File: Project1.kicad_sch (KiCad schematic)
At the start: 50 parts, among them IC1 LM324N, IC2 LM324N, IC3 LM324N, IC4 LM324N

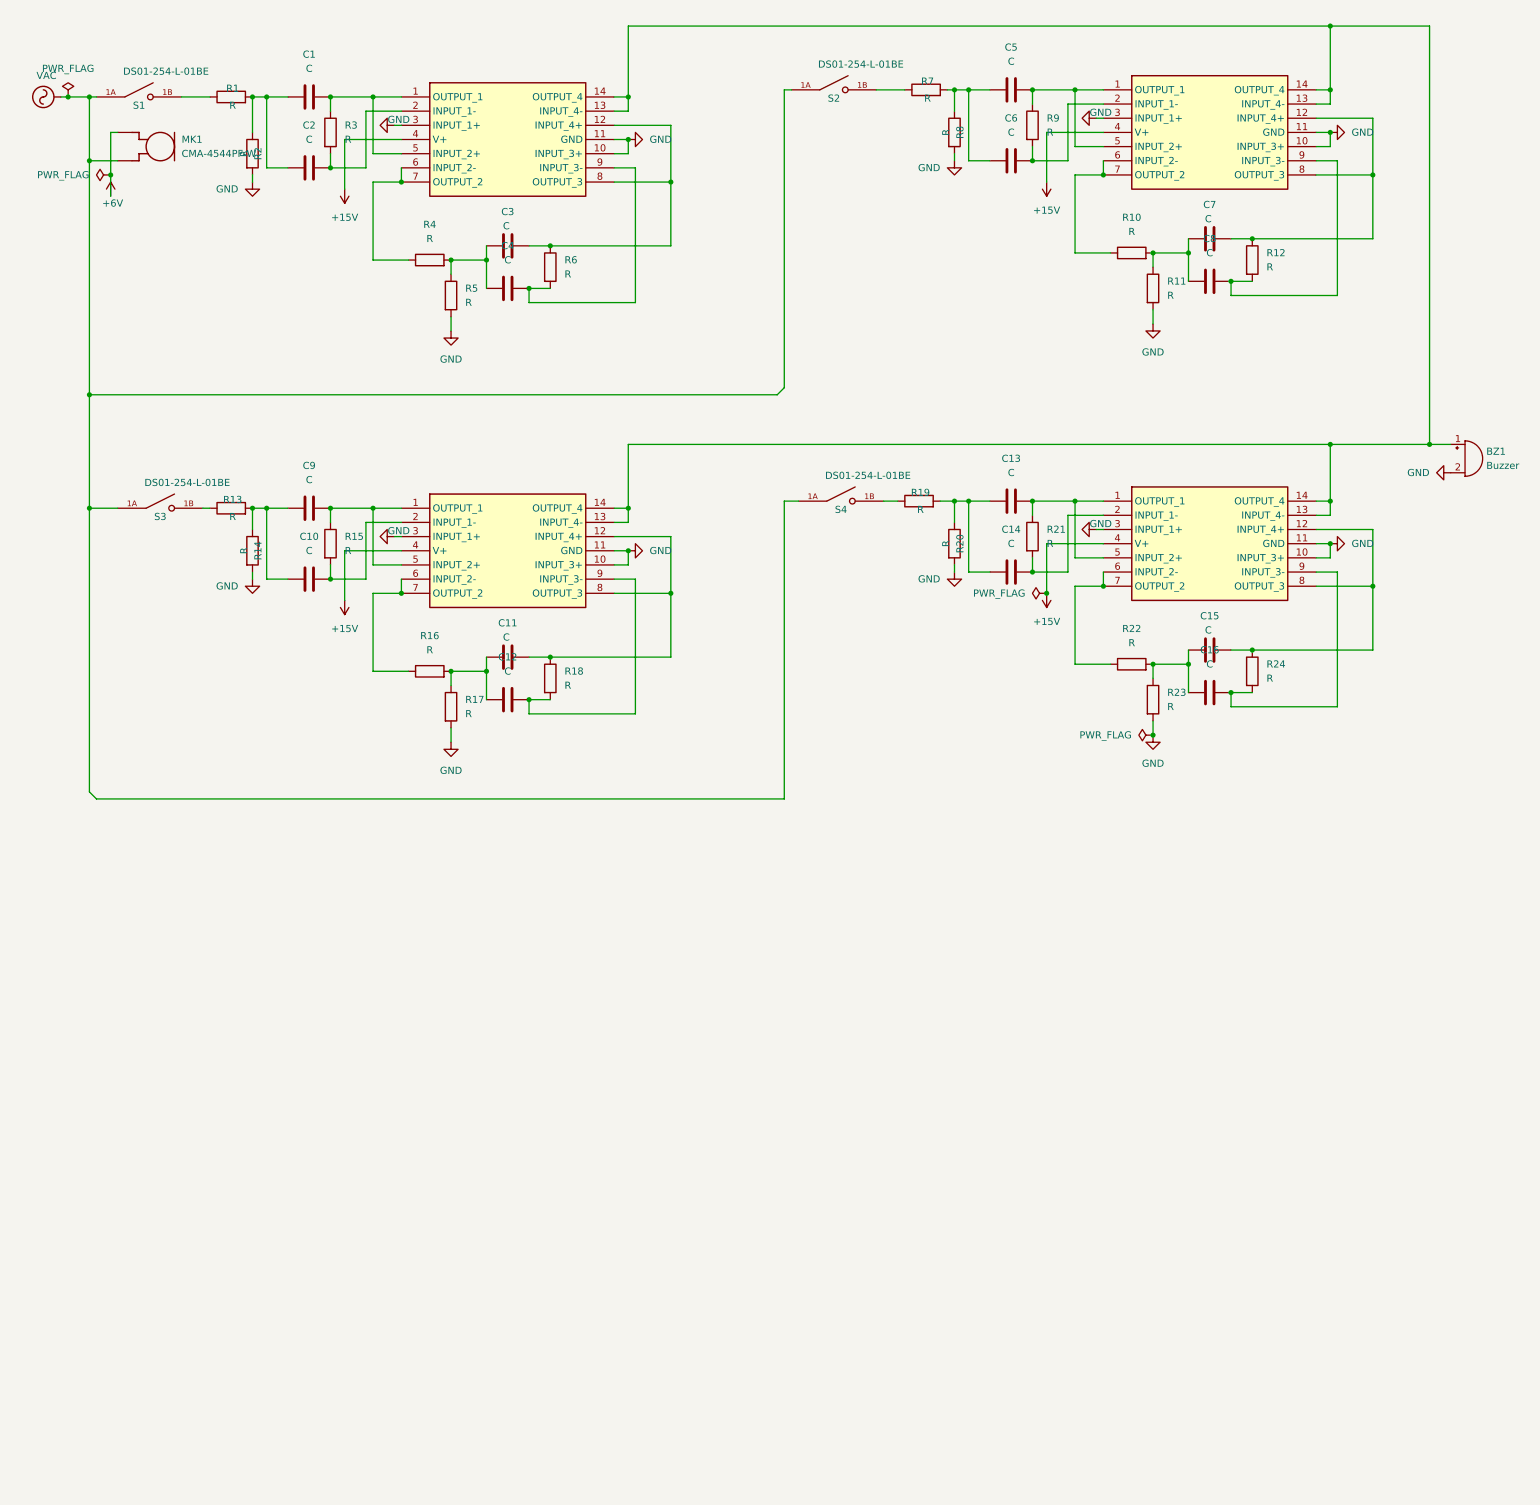
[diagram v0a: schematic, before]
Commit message: 0520 Edited.
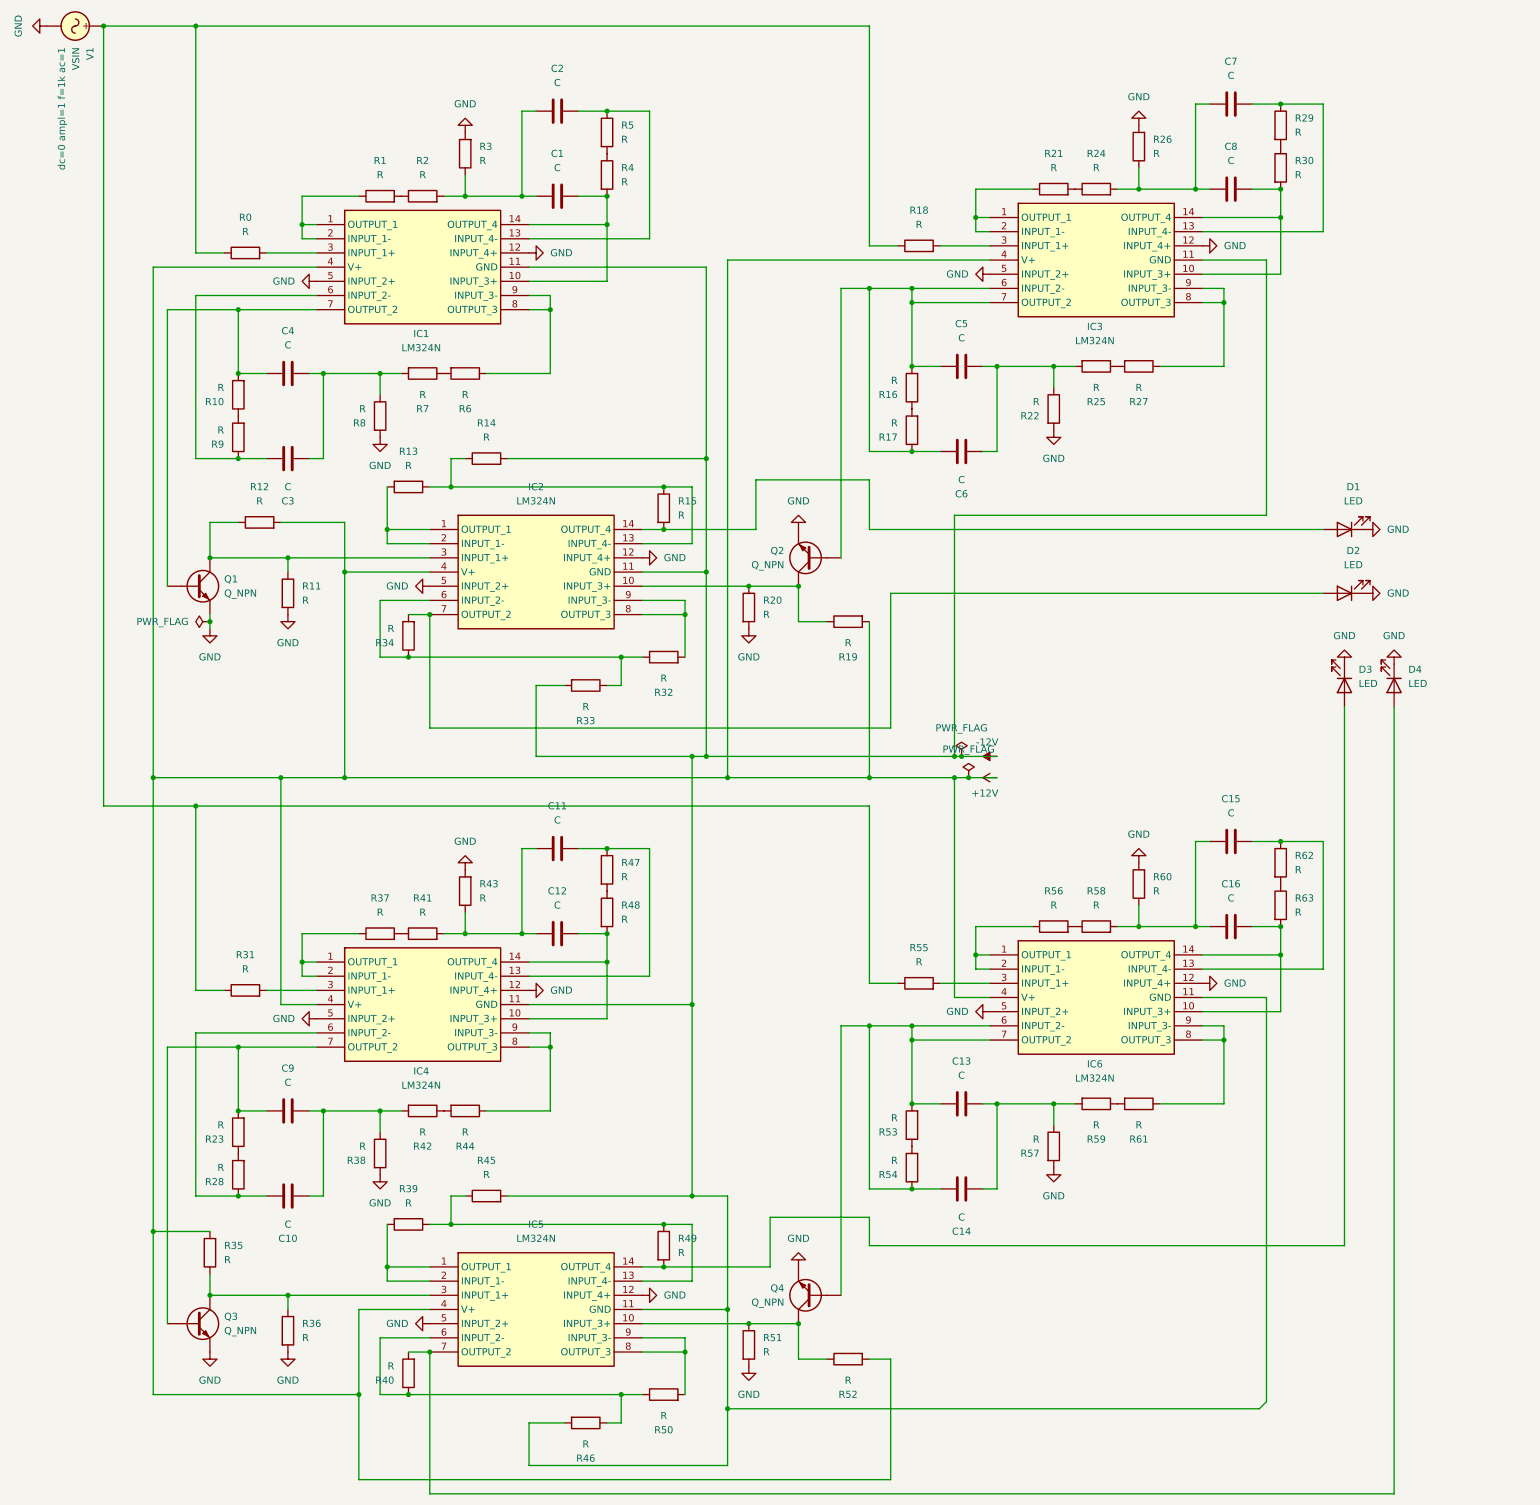
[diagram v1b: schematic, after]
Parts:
- removed BZ1: Buzzer, Buzzer_Beeper:Buzzer_12x9.5RM7.6, symbol Device:Buzzer
- removed MK1: CMA-4544PF-W, Project1:MIC_CMA-4544PF-W, symbol New_Library:CMA-4544PF-W
- removed S1, S2, S3, S4: DS01-254-L-01BE, Project1:SW_DS01-254-L-01BE, symbol New_Library:DS01-254-L-01BE
- added D1, D2, D3, D4: LED, LED_THT:LED_D3.0mm, symbol Device:LED
- added IC5, IC6: LM324N, Project1:LM324N, symbol New_Library:LM324N
- added Q1, Q2, Q3, Q4: Q_NPN, Project1:TNPN_TO-92_ONS, symbol Device:Q_NPN
- added R0, R25, R26, R27, R28, R29, R30, R31, R32, R33, R34, R35, R36, R37, R38, R39, R40, R41, R42, R43, R44, R45, R46, R47, R48, R49, R50, R51, R52, R53, R54, R55, R56, R57, R58, R59, R60, R61, R62, R63: R, Resistor_SMD:R_0603_1608Metric, symbol Device:R
- added V1: VSIN, symbol Simulation_SPICE:VSIN
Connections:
- net GND: now also IC1.12 (INPUT_4+), IC1.5 (INPUT_2+), IC2.12 (INPUT_4+), IC2.5 (INPUT_2+), IC3.12 (INPUT_4+), IC3.5 (INPUT_2+), IC4.12 (INPUT_4+), IC4.5 (INPUT_2+), R22.2, R3.2, D1.1 (K), D2.1 (K), D3.1 (K), D4.1 (K), IC5.12 (INPUT_4+), IC5.5 (INPUT_2+), IC6.12 (INPUT_4+), IC6.5 (INPUT_2+), Q1.E, Q2.E, Q3.E, Q4.E, R26.2, R36.2, R38.2, R43.2, R51.2, R57.2, R60.2, V1.2; no longer IC1.10 (INPUT_3+), IC1.11 (GND), IC1.3 (INPUT_1+), IC2.10 (INPUT_3+), IC2.11 (GND), IC2.3 (INPUT_1+), IC3.10 (INPUT_3+), IC3.11 (GND), IC3.3 (INPUT_1+), IC4.10 (INPUT_3+), IC4.11 (GND), IC4.3 (INPUT_1+), R14.2, R17.2, R2.2, R23.2, R5.2
- net at R1.2, R2.1: no longer C1.2, C2.1
- net at C13.2, C14.1: now also R57.1, R59.2; no longer R19.2, R20.1
- net at IC1.8 (OUTPUT_3), R6.1: now also IC1.9 (INPUT_3-); no longer C3.2, IC1.12 (INPUT_4+)
- net at R7.1: now also R6.2
- net at C5.2, C6.1: now also R22.1, R25.2; no longer R7.2, R8.1
- net at R16.2, R17.1: now also C5.1, C6.2, IC3.6 (INPUT_2-), IC3.7 (OUTPUT_2), Q2.B; no longer C11.1, C12.1
- net at C15.1, C16.1: now also R58.2, R60.1; no longer R22.2, R23.1
- net at R19.1: now also IC2.10 (INPUT_3+), R20.1, Q2.C
- net at R13.1: now also IC2.13 (INPUT_4-), R14.1, R15.1
- net at C10.1, C9.2: now also R38.1, R42.2; no longer R13.2, R14.1
- net at C7.1, C8.1: now also R24.2, R26.1; no longer R10.2, R11.1
- net at R1.1: now also IC1.1 (OUTPUT_1), IC1.2 (INPUT_1-)
- net at C1.1, R3.1: now also C2.1, R2.2; no longer IC1.1 (OUTPUT_1), IC1.5 (INPUT_2+)
- net +15V renamed +12V
- net +12V: now also R12.2, R19.2, IC5.4 (V+), IC6.4 (V+), R35.2, R52.2
- new net: R0.1, R18.1, R31.1, R55.1, V1.1
- new net: IC6.3 (INPUT_1+), R55.2
- new net: IC3.1 (OUTPUT_1), IC3.2 (INPUT_1-), R21.1
- new net: R21.2, R24.1
- new net: IC5.1 (OUTPUT_1), IC5.2 (INPUT_1-), R39.2
- new net: IC5.10 (INPUT_3+), Q4.C, R51.1, R52.1
- new net: IC5.13 (INPUT_4-), R39.1, R45.1, R49.1
- new net: D3.2 (A), IC5.14 (OUTPUT_4), R49.2
- new net: IC5.3 (INPUT_1+), Q3.C, R35.1, R36.1
- new net: IC5.6 (INPUT_2-), R40.1, R46.1, R50.1
- new net: D4.2 (A), IC5.7 (OUTPUT_2), R40.2
- new net: IC5.8 (OUTPUT_3), IC5.9 (INPUT_3-), R50.2
- new net: C7.2, IC3.13 (INPUT_4-), R29.1
- new net: IC2.6 (INPUT_2-), R32.1, R33.1, R34.1
- new net: R29.2, R30.1
- new net: C8.2, IC3.10 (INPUT_3+), IC3.14 (OUTPUT_4), R30.2
- new net: C2.2, IC1.13 (INPUT_4-), R5.1
- new net: R25.1, R27.2
- new net: IC2.8 (OUTPUT_3), IC2.9 (INPUT_3-), R32.2
- new net: C4.1, IC1.7 (OUTPUT_2), Q1.B, R10.2
- new net: C3.1, C4.2, R7.2, R8.1
- new net: IC6.1 (OUTPUT_1), IC6.2 (INPUT_1-), R56.1
- new net: R56.2, R58.1
- new net: IC2.1 (OUTPUT_1), IC2.2 (INPUT_1-), R13.2
- new net: D1.2 (A), IC2.14 (OUTPUT_4), R15.2
- new net: IC2.3 (INPUT_1+), Q1.C, R11.1, R12.1
- new net: D2.2 (A), IC2.7 (OUTPUT_2), R34.2
- new net: IC3.8 (OUTPUT_3), IC3.9 (INPUT_3-), R27.1
- new net: C11.1, C12.1, R41.2, R43.1
- new net: C11.2, IC4.13 (INPUT_4-), R47.1
- new net: C9.1, IC4.7 (OUTPUT_2), Q3.B, R23.2
- new net: IC3.3 (INPUT_1+), R18.2
- new net: C15.2, IC6.13 (INPUT_4-), R62.1
- new net: R53.1, R54.2
- new net: C13.1, C14.2, IC6.6 (INPUT_2-), IC6.7 (OUTPUT_2), Q4.B, R53.2, R54.1
- new net: R4.1, R5.2
- new net: C1.2, IC1.10 (INPUT_3+), IC1.14 (OUTPUT_4), R4.2
- new net: R16.1, R17.2
- new net: C12.2, IC4.10 (INPUT_3+), IC4.14 (OUTPUT_4), R48.2
- new net: IC6.8 (OUTPUT_3), IC6.9 (INPUT_3-), R61.1
- new net: R59.1, R61.2
- new net: C10.2, IC4.6 (INPUT_2-), R28.1
- new net: R47.2, R48.1
- new net: IC4.1 (OUTPUT_1), IC4.2 (INPUT_1-), R37.1
- new net: IC4.3 (INPUT_1+), R31.2
- new net: IC4.8 (OUTPUT_3), IC4.9 (INPUT_3-), R44.1
- new net: R62.2, R63.1
- new net: C16.2, IC6.10 (INPUT_3+), IC6.14 (OUTPUT_4), R63.2
- new net: C3.2, IC1.6 (INPUT_2-), R9.1
- new net: IC1.3 (INPUT_1+), R0.2
- new net: R37.2, R41.1
- new net: R23.1, R28.2
- new net: R42.1, R44.2
- new net: R10.1, R9.2
- new net -12V: IC1.11 (GND), IC2.11 (GND), IC3.11 (GND), IC4.11 (GND), IC5.11 (GND), IC6.11 (GND), R14.2, R33.2, R45.2, R46.2

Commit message: 0523 Edited.
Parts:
- removed Q1, Q2, Q3, Q4: Q_NPN, Project1:TNPN_TO-92_ONS, symbol Device:Q_NPN
- removed R0: R, Resistor_SMD:R_0603_1608Metric, symbol Device:R
- removed V1: VSIN, symbol Simulation_SPICE:VSIN
- added D5, D6, D7, D8: LED, LED_THT:LED_D3.0mm, symbol Device:LED
- added IC7: LM324N, Project1:LM324N, symbol New_Library:LM324N
- added MK1: Microphone, Project1:MIC_CMA-4544PF-W, symbol Device:Microphone
- added Q1, Q2, Q3, Q4, Q5, Q6, Q7, Q8: NPN, Project1:TO-92_FAS_NPN, symbol Simulation_SPICE:NPN
- added R64, R65, R66, R67, R68, R69, R70, R71, R72: R, Resistor_SMD:R_0201_0603Metric, symbol Device:R
- added RV1, RV10, RV11, RV12, RV13, RV14, RV15, RV16, RV2, RV3, RV4, RV5, RV6, RV7, RV8, RV9: R_Potentiometer_Trim, Project1:TRIM_TC33X-2-101E, symbol Device:R_Potentiometer_Trim
- C1, C10, C11, C12, C13, C14, C15, C16, C2, C3, C4, C5, C6, C7, C8, C9: footprint Capacitor_SMD:C_0603_1608Metric -> Capacitor_SMD:C_0201_0603Metric
- R1, R10, R11, R12, R13, R14, R15, R16, R17, R18, R19, R2, R20, R21, R22, R23, R24, R25, R26, R27, R28, R29, R3, R30, R31, R32, R33, R34, R35, R36, R37, R38, R39, R4, R40, R41, R42, R43, R44, R45, R46, R47, R48, R49, R5, R50, R51, R52, R53, R54, R55, R56, R57, R58, R59, R6, R60, R61, R62, R63, R7, R8, R9: footprint Resistor_SMD:R_0603_1608Metric -> Resistor_SMD:R_0201_0603Metric
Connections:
- net +12V: now also R11.1, R16.1, R22.1, R31.1, R37.1, R38.1, R59.1, R60.1, IC7.4 (V+); no longer R12.2, R19.2, R35.2, R52.2
- net -12V: now also R13.1, R15.1, R21.1, R28.1, R35.1, R44.1, R51.1, R56.1, IC7.11 (GND), R65.2, R67.2; no longer R14.2, R33.2, R45.2, R46.2
- net GND: now also IC1.10 (INPUT_3+), IC1.3 (INPUT_1+), IC2.3 (INPUT_1+), IC3.3 (INPUT_1+), IC4.3 (INPUT_1+), IC5.10 (INPUT_3+), IC5.3 (INPUT_1+), IC6.3 (INPUT_1+), R10.2, R18.2, R24.2, R30.2, R42.2, R54.2, R55.2, D5.1 (K), D6.1 (K), D7.1 (K), D8.1 (K), IC7.10 (INPUT_3+), IC7.12 (INPUT_4+), IC7.5 (INPUT_2+), Q1.3 (E), Q2.3 (E), Q3.3 (E), Q4.3 (E), Q5.3 (E), Q6.3 (E), Q7.3 (E), Q8.3 (E), R69.1, RV1.1, RV2.1, RV3.1, RV4.1, RV5.1, RV6.1, RV7.1, RV8.1; no longer IC2.5 (INPUT_2+), IC3.5 (INPUT_2+), IC4.5 (INPUT_2+), IC6.5 (INPUT_2+), R11.2, R20.2, R22.2, R26.2, R3.2, R36.2, R38.2, R51.2, R57.2, R60.2, R8.2
- net at R21.2: now also IC4.2 (INPUT_1-), R23.1, R25.1; no longer R24.1
- net at IC5.2 (INPUT_1-), R39.2: now also C10.2; no longer IC5.1 (OUTPUT_1)
- net at C7.1, C8.1: now also R7.2, RV4.2; no longer R24.2, R26.1
- net at R33.1, R34.1: now also R1.1, R3.1, R5.1, R63.1, R7.1, IC7.13 (INPUT_4-), R64.1, R71.1; no longer IC2.6 (INPUT_2-), R32.1
- net at R29.2: now also IC4.14 (OUTPUT_4), D8.2 (A); no longer R30.1
- net at C1.1, C2.1: now also R1.2, RV1.2; no longer R2.2, R3.1
- net at R27.2: now also RV11.3; no longer R25.1
- net at IC2.8 (OUTPUT_3), IC2.9 (INPUT_3-): now also R19.2; no longer R32.2
- net at R58.1: now also C16.2, IC5.8 (OUTPUT_3), RV16.2; no longer R56.2
- net at IC2.2 (INPUT_1-), R13.2: now also R12.1, R14.1; no longer IC2.1 (OUTPUT_1)
- net at IC3.8 (OUTPUT_3), IC3.9 (INPUT_3-): now also R46.2; no longer R27.1
- net at C15.1, C16.1: now also R64.2, RV8.2; no longer R58.2, R60.1
- net at R6.2: now also C6.2, IC1.13 (INPUT_4-); no longer R7.1
- net at C11.1, C12.1: now also R34.2, RV6.2; no longer R41.2, R43.1
- net at R2.1: now also C2.2, IC1.1 (OUTPUT_1), RV9.2; no longer R1.2
- net at R53.1: now also IC6.13 (INPUT_4-), R51.2, R52.1; no longer R54.2
- net at R5.2: now also C5.1, C6.1, RV3.2; no longer R4.1
- net at R17.2: now also D4.2 (A), IC2.14 (OUTPUT_4); no longer R16.1
- net at IC6.8 (OUTPUT_3), IC6.9 (INPUT_3-): now also R53.2; no longer R61.1
- net at R61.2: now also IC6.1 (OUTPUT_1), D6.2 (A); no longer R59.1
- net at C13.2, R57.1: now also IC5.14 (OUTPUT_4), RV14.2; no longer C14.1, R59.2
- net at R47.2: now also RV13.3; no longer R48.1
- net at R31.2: now also IC3.5 (INPUT_2+), R30.1, Q4.1 (C); no longer IC4.3 (INPUT_1+)
- net at IC4.8 (OUTPUT_3), IC4.9 (INPUT_3-): now also R32.2; no longer R44.1
- net at R62.2: now also IC6.6 (INPUT_2-), IC6.7 (OUTPUT_2); no longer R63.1
- net at R37.2: now also IC4.5 (INPUT_2+), R42.1, Q5.1 (C); no longer R41.1
- net at R28.2: now also IC4.13 (INPUT_4-), R29.1, R32.1; no longer R23.1
- net at R44.2: now also IC3.13 (INPUT_4-), R45.1, R46.1; no longer R42.1
- net at R10.1: now also IC2.5 (INPUT_2+), R11.2, Q1.1 (C); no longer R9.2
- new net: R50.2, RV16.3
- new net: R9.2, RV9.3
- new net: C9.2, IC5.1 (OUTPUT_1), R39.1, RV13.2
- new net: C14.2, IC5.13 (INPUT_4-), R57.2
- new net: C11.2, IC5.6 (INPUT_2-), R40.2
- new net: C12.2, IC5.7 (OUTPUT_2), R40.1, RV15.2
- new net: C15.2, IC5.9 (INPUT_3-), R58.2
- new net: IC6.5 (INPUT_2+), Q6.1 (C), R38.2, R43.1
- new net: IC3.2 (INPUT_1-), R35.2, R36.1, R41.1
- new net: D2.2 (A), IC3.1 (OUTPUT_1), R36.2
- new net: C13.1, C14.1, R63.2, RV7.2
- new net: IC7.3 (INPUT_1+), MK1.1 (-), R69.2
- new net: C10.1, C9.1, R33.2, RV5.2
- new net: C5.2, IC1.14 (OUTPUT_4), R6.1, RV10.2
- new net: C7.2, IC1.8 (OUTPUT_3), R8.1, RV12.2
- new net: IC6.10 (INPUT_3+), Q8.1 (C), R55.1, R60.2
- new net: IC6.2 (INPUT_1-), R56.2, R61.1, R62.1
- new net: IC7.7 (OUTPUT_2), R70.2, R72.1
- new net: IC7.14 (OUTPUT_4), R71.2, R72.2
- new net: Q8.2 (B), R50.1
- new net: Q7.2 (B), R49.1
- new net: R49.2, RV14.3
- new net: IC7.1 (OUTPUT_1), IC7.2 (INPUT_1-), R68.2
- new net: IC7.6 (INPUT_2-), R67.1, R68.1, R70.1
- new net: IC7.8 (OUTPUT_3), MK1.2 (+), R66.2
- new net: IC7.9 (INPUT_3-), R65.1, R66.1
- new net: C3.2, IC1.7 (OUTPUT_2), R4.1, RV11.2
- new net: C3.1, C4.1, R3.2, RV2.2
- new net: C4.2, IC1.6 (INPUT_2-), R4.2
- new net: IC4.10 (INPUT_3+), Q7.1 (C), R54.1, R59.2
- new net: IC4.6 (INPUT_2-), IC4.7 (OUTPUT_2), R25.2
- new net: IC2.13 (INPUT_4-), R15.2, R17.1, R19.1
- new net: IC2.10 (INPUT_3+), Q2.1 (C), R16.2, R18.1
- new net: D5.2 (A), IC4.1 (OUTPUT_1), R23.2
- new net: D7.2 (A), IC6.14 (OUTPUT_4), R52.2
- new net: D1.2 (A), IC2.1 (OUTPUT_1), R14.2
- new net: Q6.2 (B), R48.1
- new net: R48.2, RV15.3
- new net: Q3.2 (B), R26.1
- new net: R26.2, RV12.3
- new net: Q2.2 (B), R20.1
- new net: D3.2 (A), IC3.14 (OUTPUT_4), R45.2
- new net: Q1.2 (B), R9.1
- new net: IC3.6 (INPUT_2-), IC3.7 (OUTPUT_2), R41.2
- new net: C1.2, IC1.2 (INPUT_1-), R2.2
- new net: IC3.10 (INPUT_3+), Q3.1 (C), R22.2, R24.1
- new net: R20.2, RV10.3
- new net: Q4.2 (B), R27.1
- new net: C8.2, IC1.9 (INPUT_3-), R8.2
- new net: Q5.2 (B), R47.1
- new net: IC2.6 (INPUT_2-), IC2.7 (OUTPUT_2), R12.2
- no-connect marks 0 -> 16
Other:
- note added: "-12V"
- note added: "-12V power"
- note added: "12V power"
